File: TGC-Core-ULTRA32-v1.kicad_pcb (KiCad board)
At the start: 4 copper layers, 38.8 x 59 mm, 32 parts, among them J1 Conn_01x19, J2 Conn_01x19, P1 USB_C_Plug_USB2.0, Q1 SS8050-G, Q2 SS8050-G, SW1 SW_Push, SW2 SW_Push, U1 CP2102N-Axx-xQFN28, U2 AMS1117-3.3

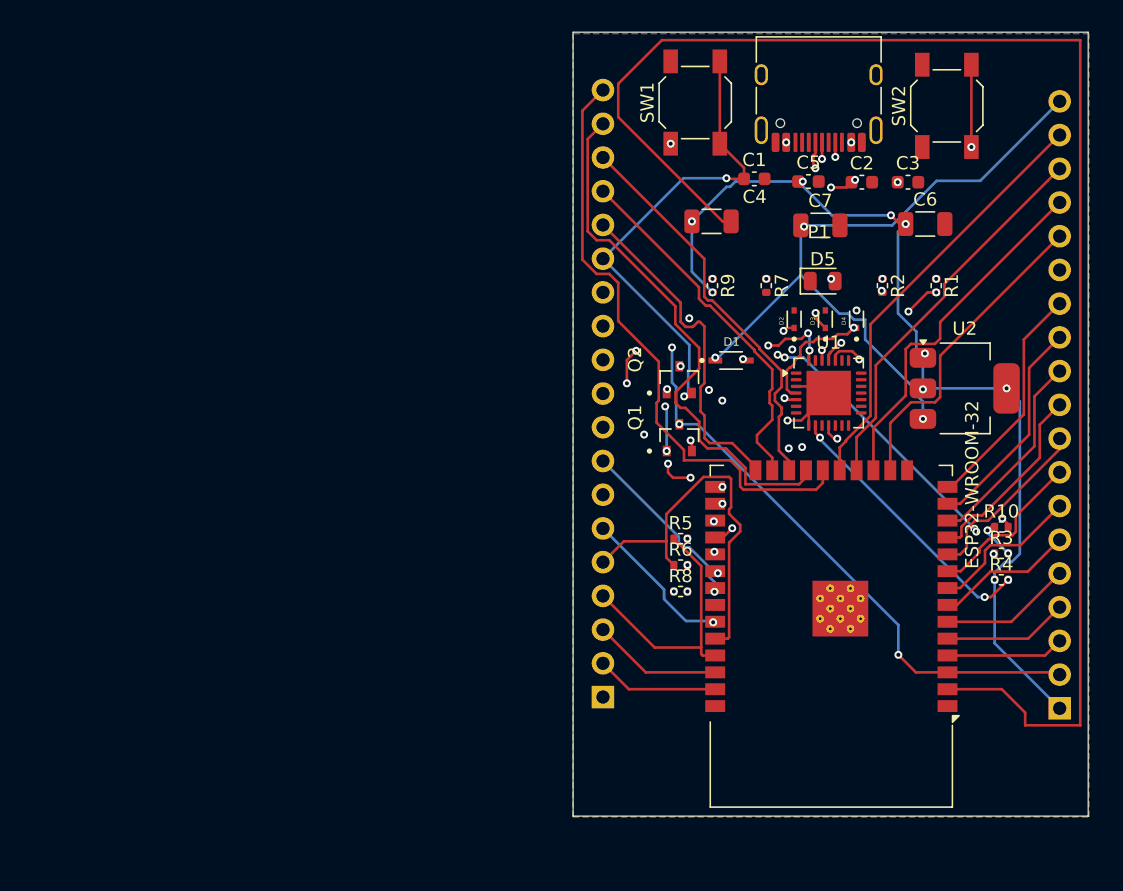
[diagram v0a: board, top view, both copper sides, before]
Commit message: Add files via upload
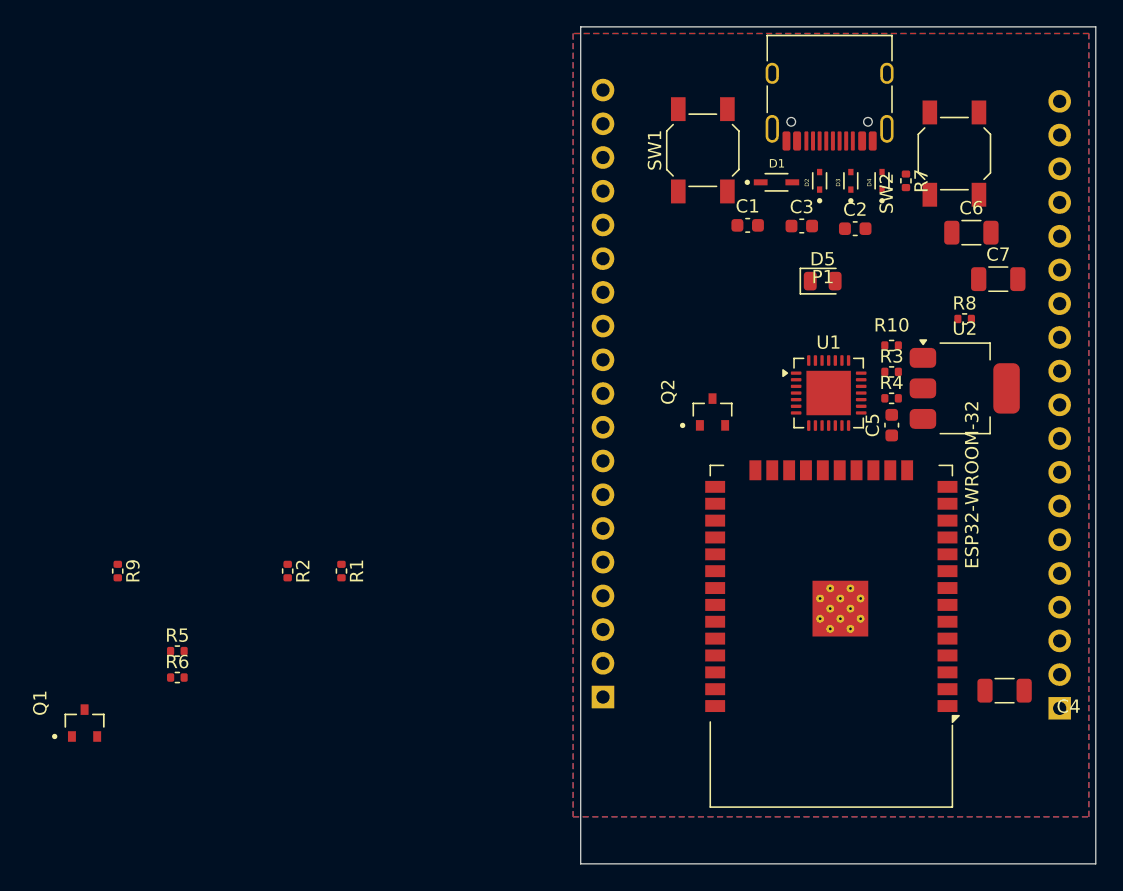
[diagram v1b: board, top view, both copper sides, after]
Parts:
- moved Q1 49.7 mm to (63.7, 175.4)
- moved R1 49.7 mm to (83.0, 164.0)
- moved R2 49.7 mm to (79.0, 164.0)
- moved R9 49.7 mm to (66.2, 164.0)
- moved C4 41.7 mm to (133.0, 173.0)
- moved R5 38.8 mm to (70.7, 170.0)
- moved R6 38.8 mm to (70.7, 172.0)
- moved R8 29.6 mm to (130.0, 145.0)
- moved C5 19.4 mm to (124.5, 153.0), turned to 90 degrees
- moved R4 16.0 mm to (124.5, 151.0)
- moved R10 16.0 mm to (124.5, 147.0)
- moved R3 16.0 mm to (124.5, 149.0)
- moved C7 14.0 mm to (132.5, 142.0)
- moved D1 13.9 mm to (115.8, 134.7)
- moved R7 13.2 mm to (125.6, 134.6)
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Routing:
- net Net-(ESP32-WROOM-32-VDD): track 113.7 -> 0.00 mm
- net +5V: track 90.1 -> 0.00 mm, vias 4 -> 0
- net /EN: track 79.8 -> 0.00 mm, vias 9 -> 0
- net +3.3V: track 72.3 -> 0.00 mm, vias 8 -> 0
- net /VBUS: track 48.1 -> 0.00 mm, vias 8 -> 0
- net /IO0: track 47.3 -> 0.00 mm, vias 3 -> 0
- net /CLK: track 45.6 -> 0.00 mm
- net GND: track 45.4 -> 0.00 mm, vias 7 -> 0
- net Net-(D5-Pad2): track 45.2 -> 0.00 mm, vias 2 -> 0
- net /SD0: track 40.9 -> 0.00 mm
- net /IO18: track 37.9 -> 0.00 mm, vias 1 -> 0
- net /IO5: track 37.0 -> 0.00 mm, vias 1 -> 0
- net /IO4: track 35.3 -> 0.00 mm, vias 5 -> 0
- net /RTS: track 35.1 -> 0.00 mm, vias 5 -> 0
- net /D+: track 32.7 -> 0.00 mm, vias 2 -> 0
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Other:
- board size 38.8 x 59 mm -> 38.8 x 63 mm
